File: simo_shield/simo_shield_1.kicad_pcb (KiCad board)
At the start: 2 copper layers, 70 x 100 mm, 11 parts, among them J1 Conn_01x02_Female, J2 Conn_01x02_Female, J3 Conn_01x01_Female, U1 elemon_board, U2 modulo_flash_externa, U3 bluepill_board_stm32, U4 modulo_acelerometro

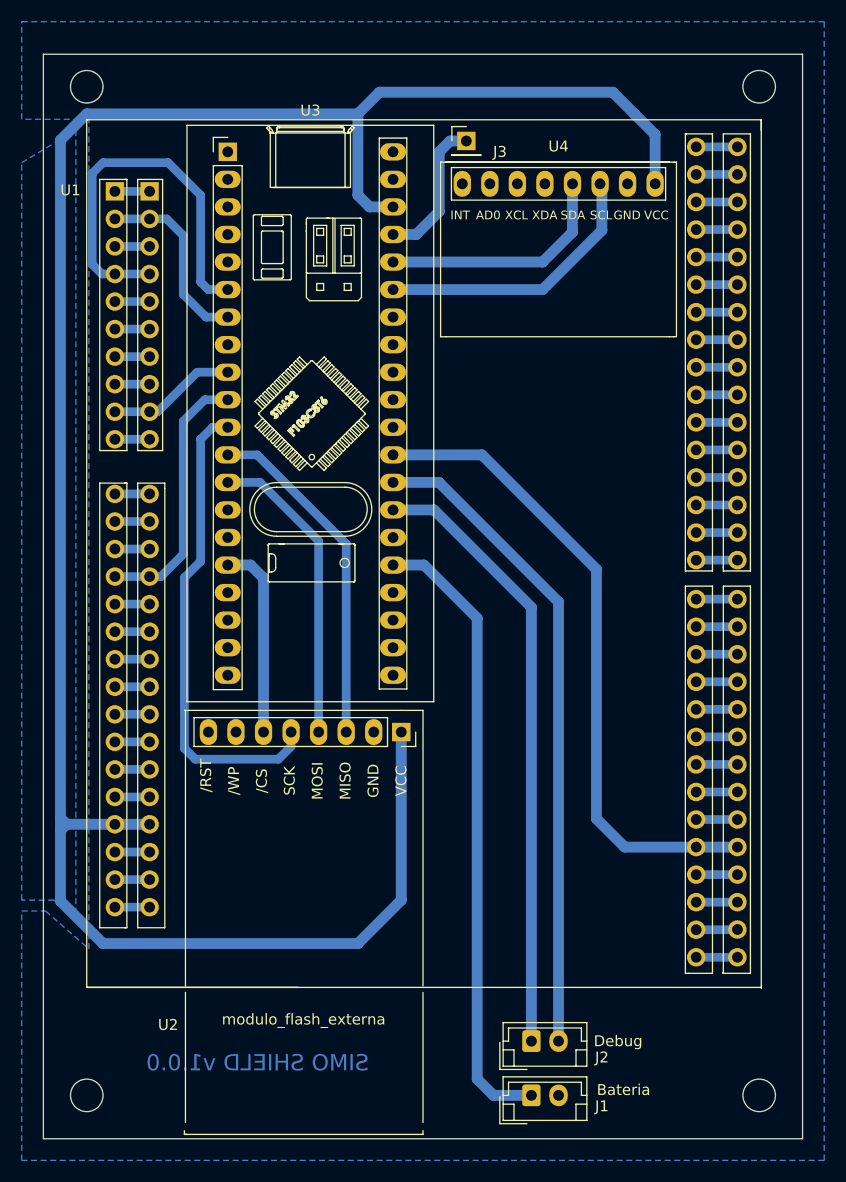
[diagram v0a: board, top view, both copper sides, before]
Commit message: update pcb
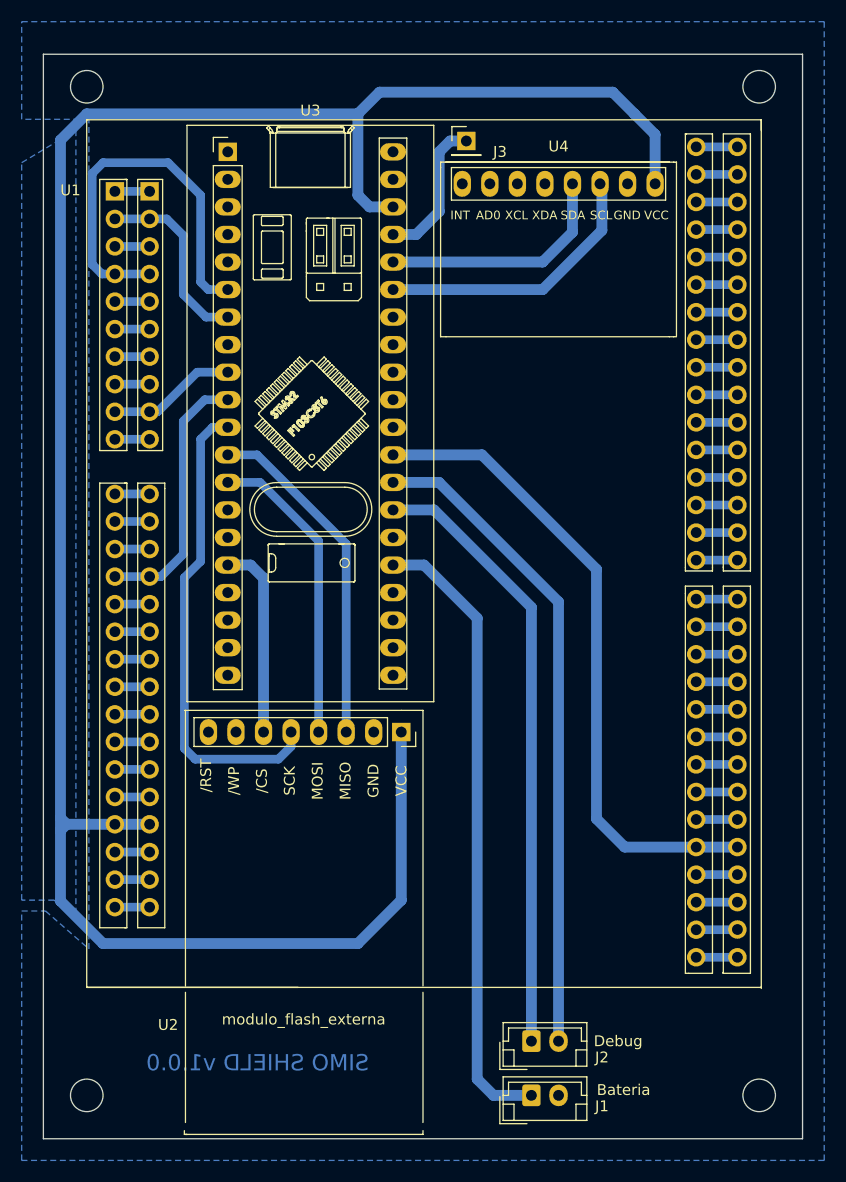
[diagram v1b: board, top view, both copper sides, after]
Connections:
- U4 pad 7: +3.3V -> GND
- U4 pad 8: GND -> +3.3V
